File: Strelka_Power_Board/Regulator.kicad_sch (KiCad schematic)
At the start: 24 parts

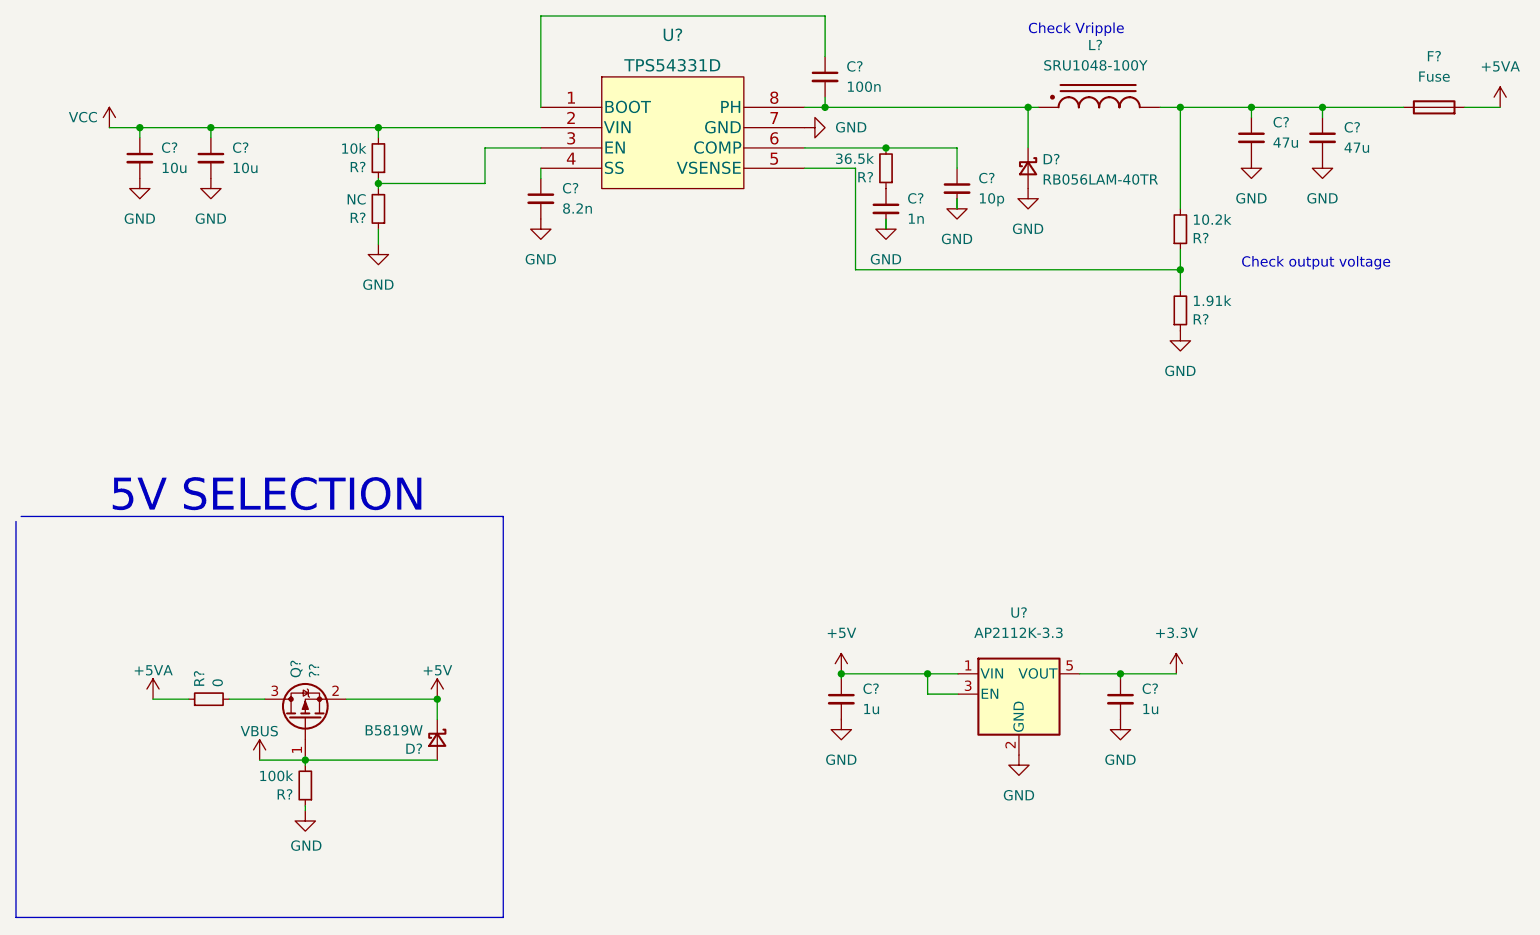
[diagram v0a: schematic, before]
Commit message: Creating BOM
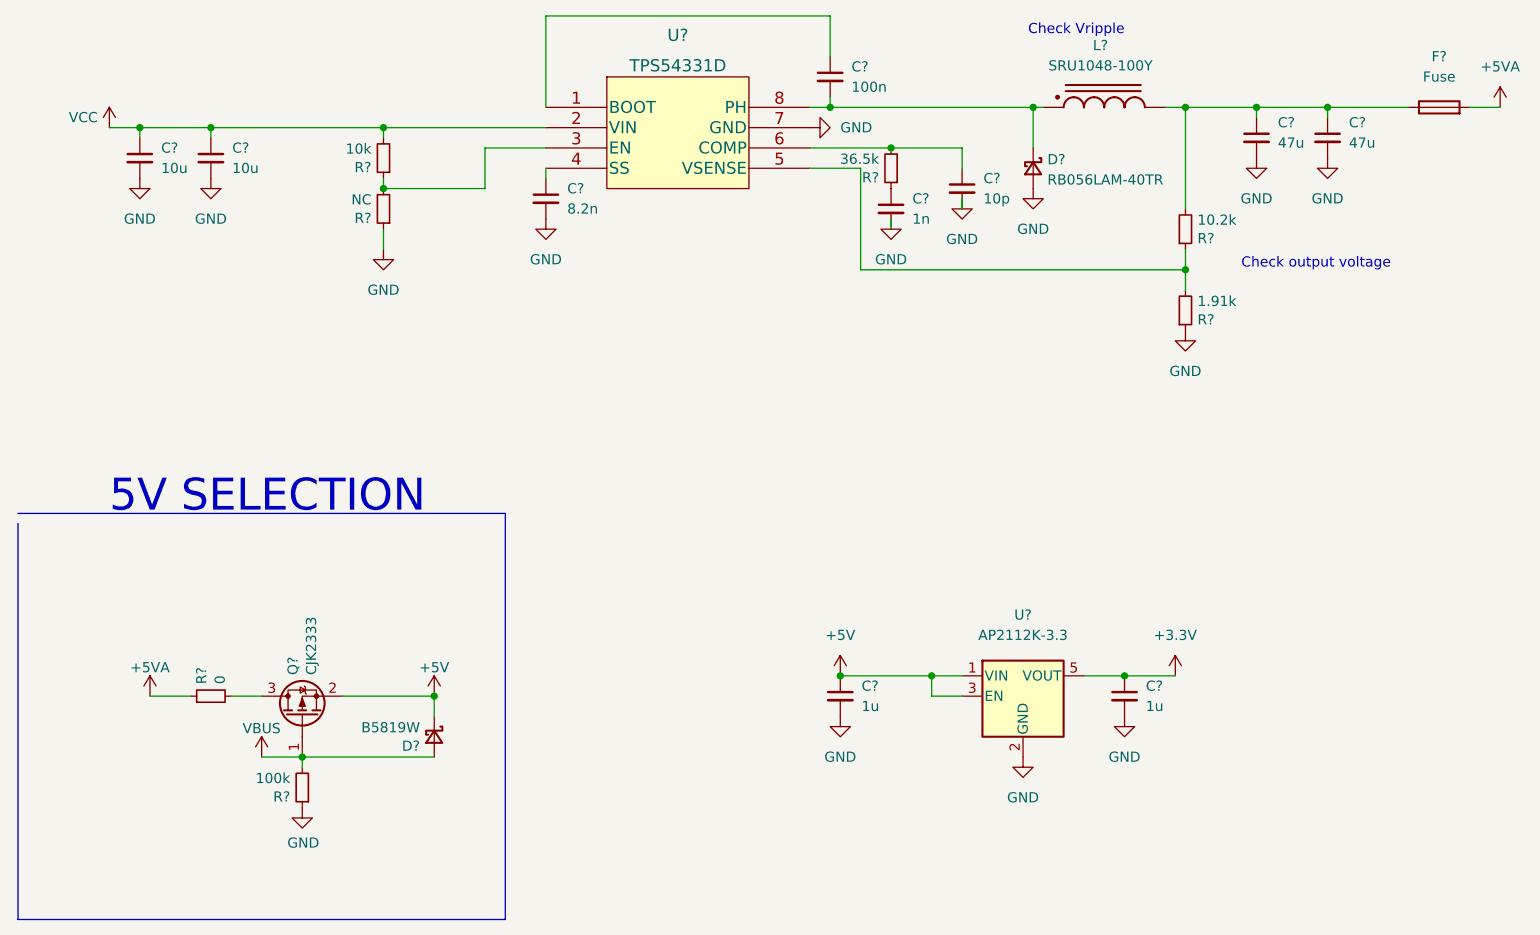
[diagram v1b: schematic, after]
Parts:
- removed C?: 47u, Capacitor_SMD:C_0603_1608Metric, symbol Device:C_Small
- removed Q?: ??, Package_TO_SOT_SMD:SOT-23, symbol Transistor_FET:Si2319CDS
- added C?: 47u, Capacitor_SMD:C_0805_2012Metric, symbol Device:C_Small
- added Q?: CJK2333, Package_TO_SOT_SMD:SOT-23, symbol Transistor_FET:Si2319CDS
- C?: footprint Capacitor_SMD:C_0603_1608Metric -> Capacitor_SMD:C_0805_2012Metric
- D?: LCSC# (none) -> C3760036
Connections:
- net +5V: now also Q?.2 (S)
- net GND: now also C?.2
- net VBUS: now also Q?.1 (G)
- net at C?.1, F?.1, L?.2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: now also C?.1
- net at R?.2: now also Q?.3 (D)
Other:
- moved on the sheet: C?, D?, F?, L?, R?, U?

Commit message: redo placement
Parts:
- L?: MANUFACTURER Bourns -> (none); MAXIMUM_PACKAGE_HEIGHT 5.1mm -> (none); PARTREV 03/18 -> (none); STANDARD Manufacturer Recommendations -> (none)
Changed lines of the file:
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@@
-      (effects (font (size 1.27 1.27)) (justify left bottom) hide)
-    )
-    (property "STANDARD" "Manufacturer Recommendations" (id 4) (at 190.5 41.91 0)
-      (effects (font (size 1.27 1.27)) (justify left bottom) hide)
-    )
-    (property "PARTREV" "03/18" (id 5) (at 190.5 41.91 0)
-      (effects (font (size 1.27 1.27)) (justify left bottom) hide)
-    )
-    (property "MANUFACTURER" "Bourns" (id 6) (at 190.5 41.91 0)
-      (effects (font (size 1.27 1.27)) (justify left bottom) hide)
-    )
-    (property "MAXIMUM_PACKAGE_HEIGHT" "5.1mm" (id 7) (at 190.5 41.91 0)
       (effects (font (size 1.27 1.27)) (justify left bottom) hide)
     )
